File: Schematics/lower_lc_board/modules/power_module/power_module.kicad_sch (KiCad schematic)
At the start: 34 parts, among them J1 Stack Male Edge Connector, U1 TVS3300DRV, U10 ID_LM66100DCKR, U2 AMS1117, U3 ID_LM66100DCKR, U4 ID_LM66100DCKR

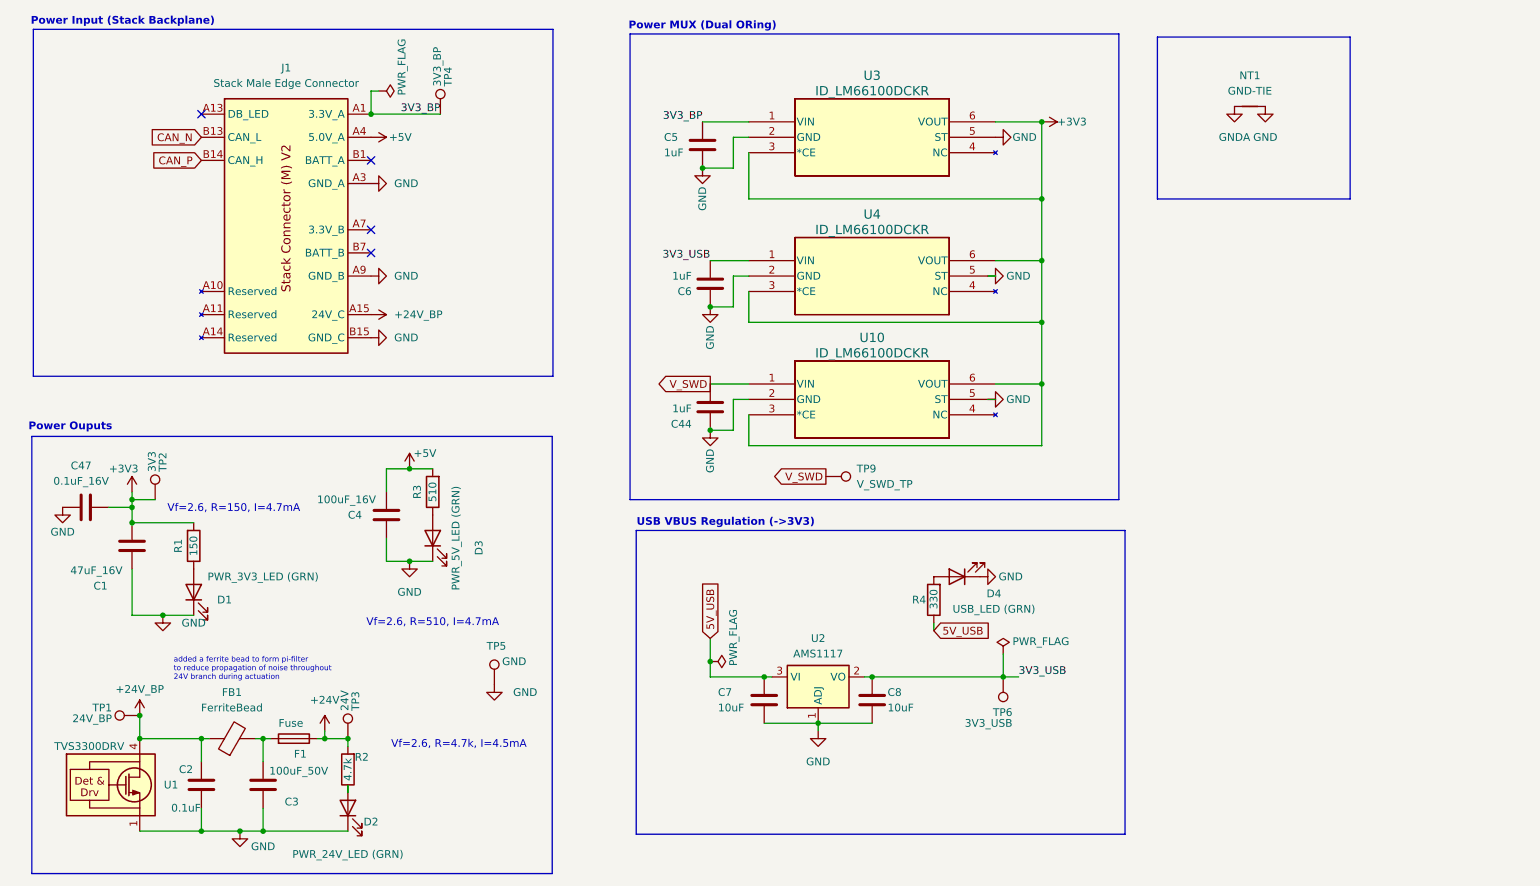
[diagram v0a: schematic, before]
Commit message: organizational work
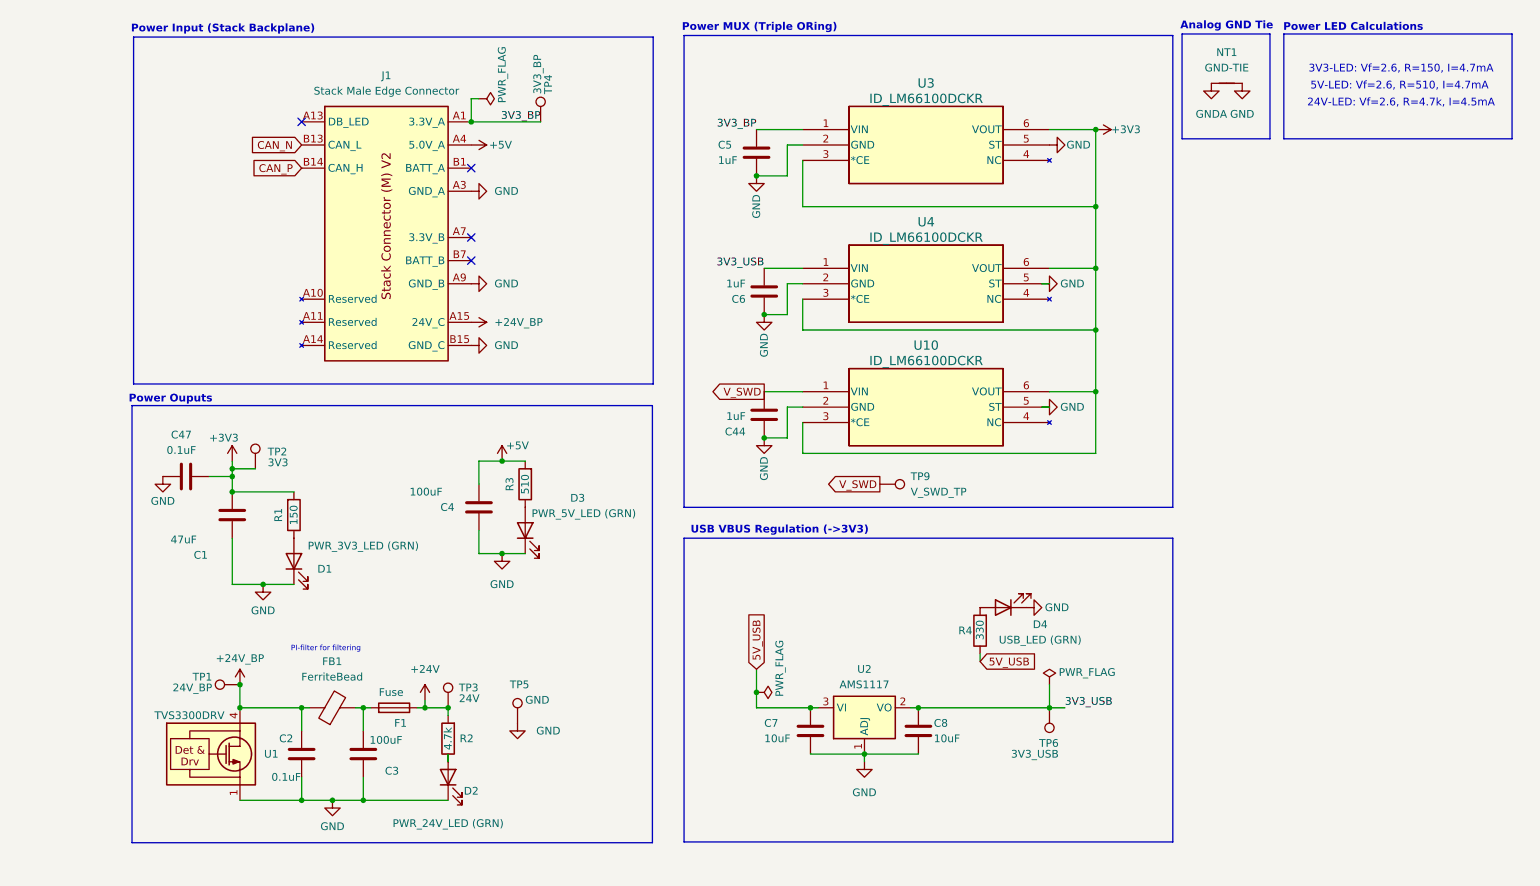
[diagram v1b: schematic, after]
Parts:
- C1: value 47uF_16V -> 47uF
- C2: JLCPCB (none) -> C14663
- C3: value 100uF_50V -> 100uF
- C4: value 100uF_16V -> 100uF
- C44, C5, C6: JLCPCB (none) -> C15849
- C47: value 0.1uF_16V -> 0.1uF
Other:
- note added: "24V-LED: Vf=2.6, R=4.7k, I=4.5mA"
- note added: "3V3-LED: Vf=2.6, R=150, I=4.7mA"
- note added: "5V-LED: Vf=2.6, R=510, I=4.7mA"
- note added: "Analog GND Tie"
- note added: "PI-filter for filtering"
- note added: "Power LED Calculations"
- note added: "Power MUX (Triple ORing)"
- note removed: "Power MUX (Dual ORing)"
- note removed: "Vf=2.6, R=150, I=4.7mA"
- note removed: "Vf=2.6, R=4.7k, I=4.5mA"
- note removed: "Vf=2.6, R=510, I=4.7mA"
- note removed: "added a ferrite bead to form pi-filter to reduce propagation of noise throughout 24V branch during actuation"
- moved on the sheet: C1, C2, C3, C4, C44, C47, C5, C6, C7, C8, D1, D2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
